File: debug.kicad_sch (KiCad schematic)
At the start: 65 parts, among them J701 USB4105-GF-A, J702 2x10 pin IDC, U701 USBLC6-2SC6, U702 FT231XQ-R, U703 TCA9554PW

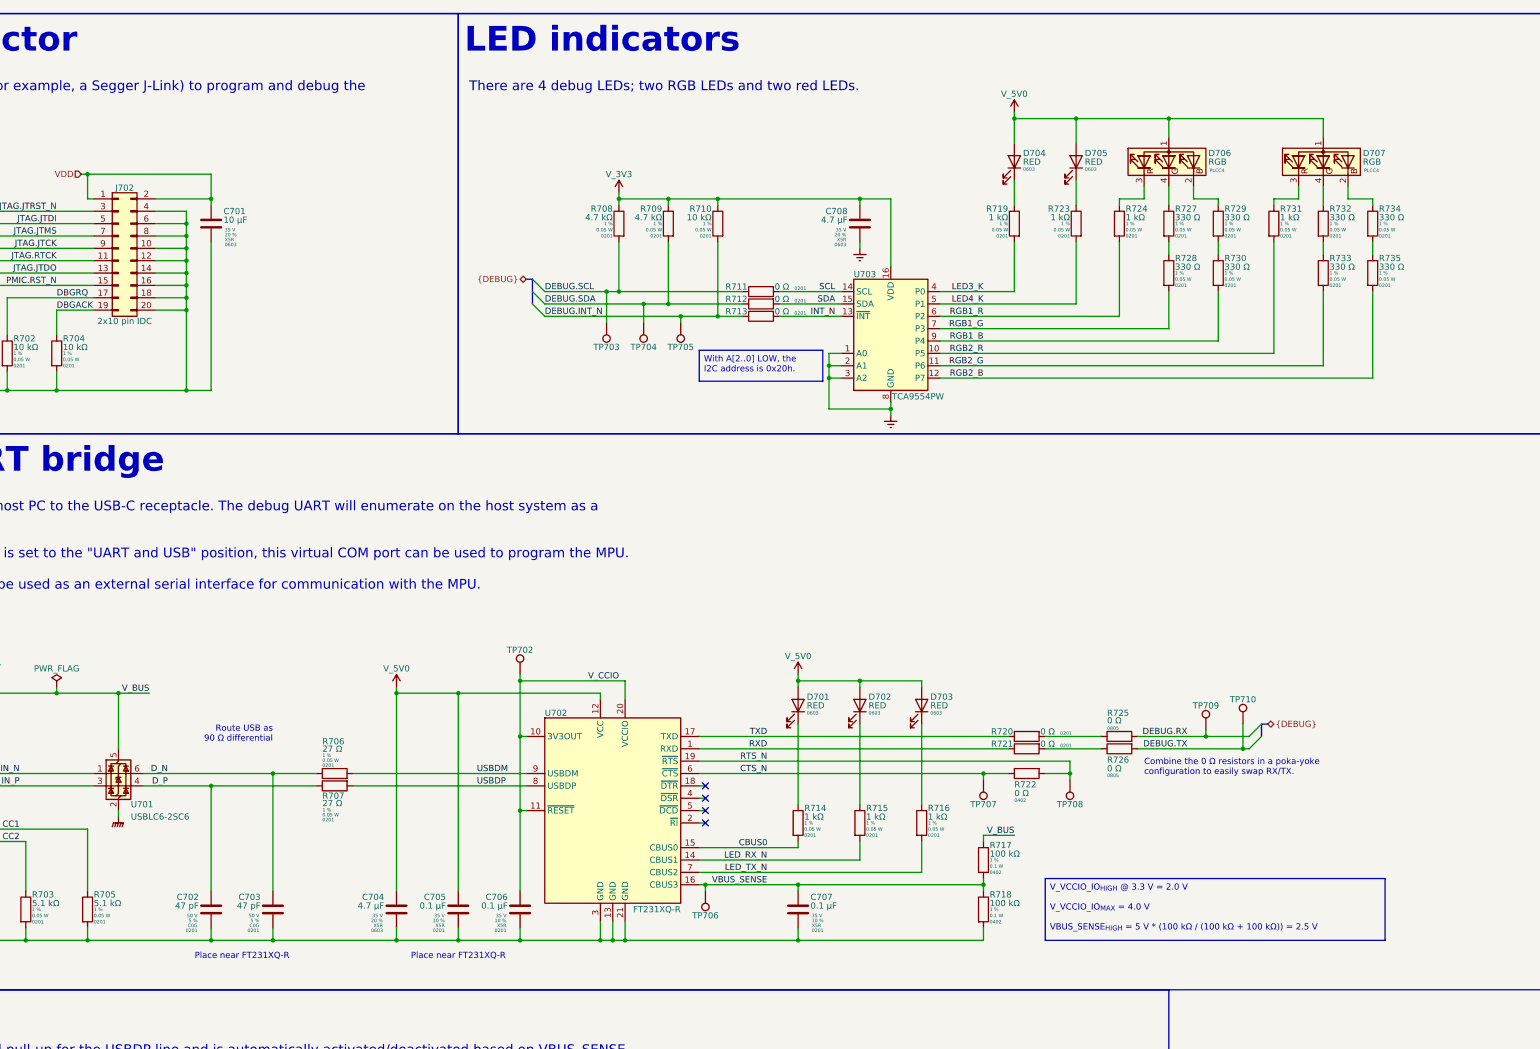
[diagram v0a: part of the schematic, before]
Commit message: Clean up schematics
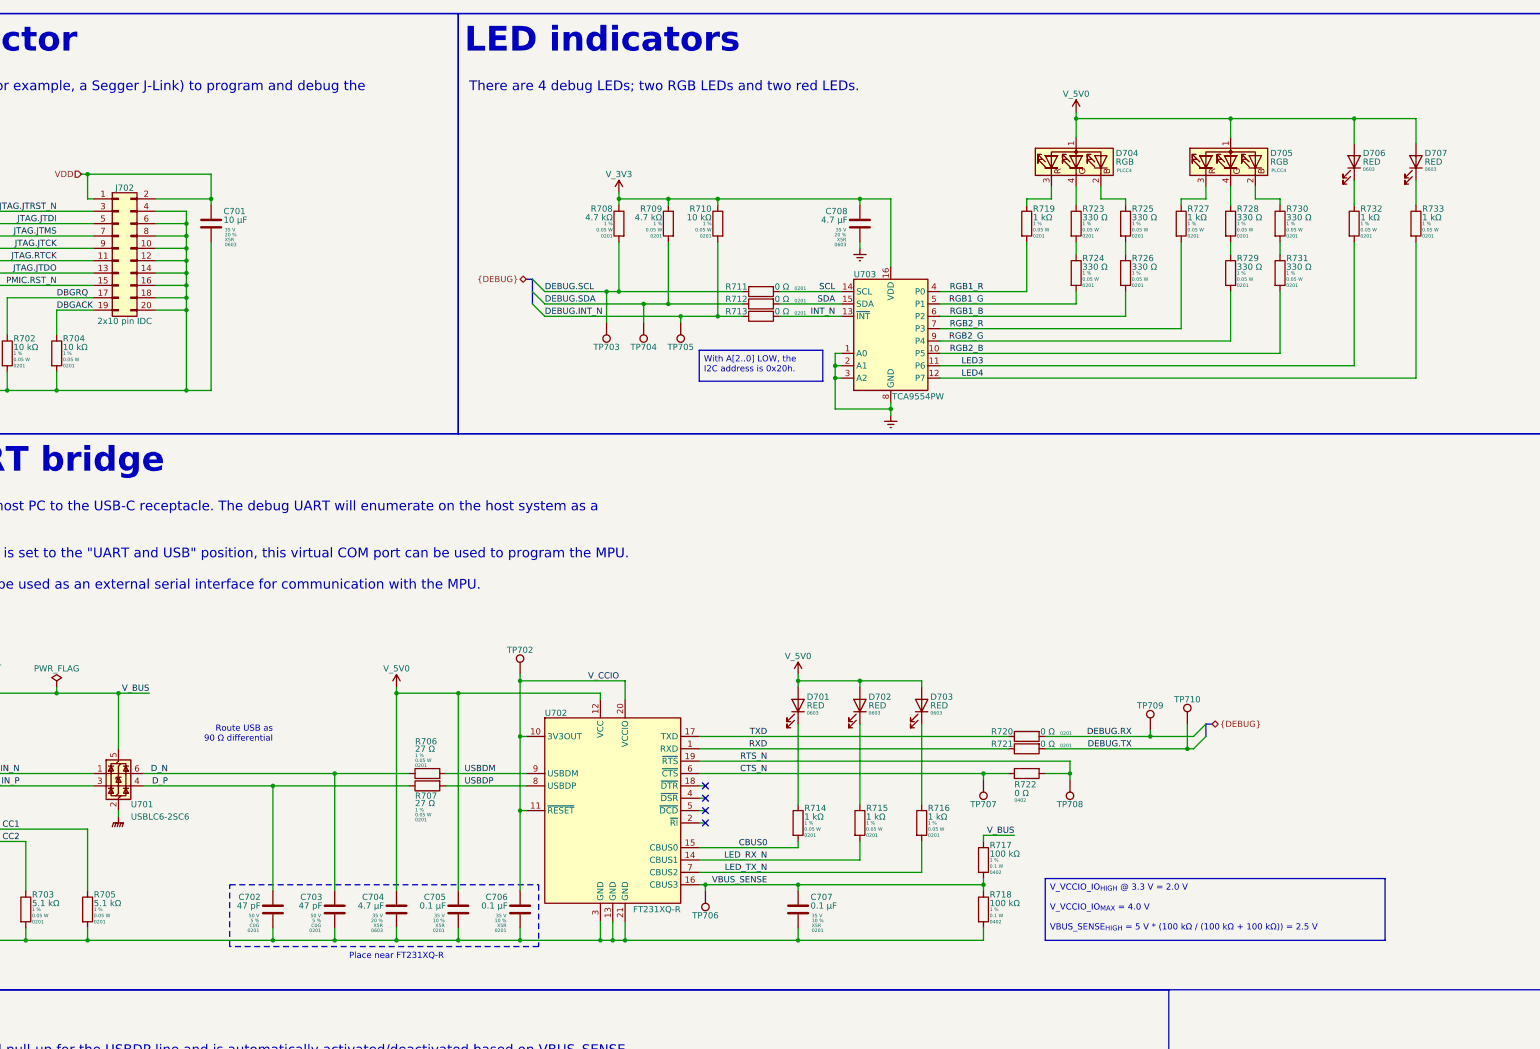
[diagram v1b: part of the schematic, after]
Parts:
- removed R725, R726: 0 Ω, Resistor_SMD:R_0805_2012Metric, symbol Device:R
- renumbered D706 to D704, D707 to D705, D704 to D706, D705 to D707, R724 to R719, R727 to R723, R728 to R724, R729 to R725, R730 to R726, R731 to R727, R732 to R728, R733 to R729, R734 to R730, R735 to R731, R719 to R732, R723 to R733
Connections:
- net DEBUG.RX: now also R720.2
- net DEBUG.TX: now also R721.2
- net RGB1_B: now also U703.6 (P2); no longer U703.9 (P4)
- net RGB1_G: now also U703.5 (P1); no longer U703.7 (P3)
- net RGB1_R: now also U703.4 (P0); no longer U703.6 (P2)
- net RGB2_B: now also U703.10 (P5); no longer U703.12 (P7)
- net RGB2_G: now also U703.9 (P4); no longer U703.11 (P6)
- net RGB2_R: now also U703.7 (P3); no longer U703.10 (P5)
- net LED3_K renamed LED3
- net LED3: now also U703.11 (P6); no longer U703.4 (P0)
- net LED4_K renamed LED4
- net LED4: now also U703.12 (P7); no longer U703.5 (P1)
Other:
- note removed: "Combine the 0 Ω resistors in a poka-yoke configuration to easily swap RX/TX."
- moved on the sheet: C702, C703, D704, D705, D706, D707, R706, R707, R719, R723, R724, R725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
